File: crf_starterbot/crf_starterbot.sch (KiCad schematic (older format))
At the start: 49 parts, among them J101 Screw_Terminal_01x02, J102 Conn_01x10_Female, J103 Screw_Terminal_01x02, J104 Screw_Terminal_01x02, Q101 Q_NPN_BCE, SW101 SW_SPST, SW102 SW_SPST, SW103 SW_SPST, U101 WeMos_D1_mini, U102 HC-SR04, U103 LM393, U104 E048-03, U106 E048-03, U107 L9110, U108 L9110

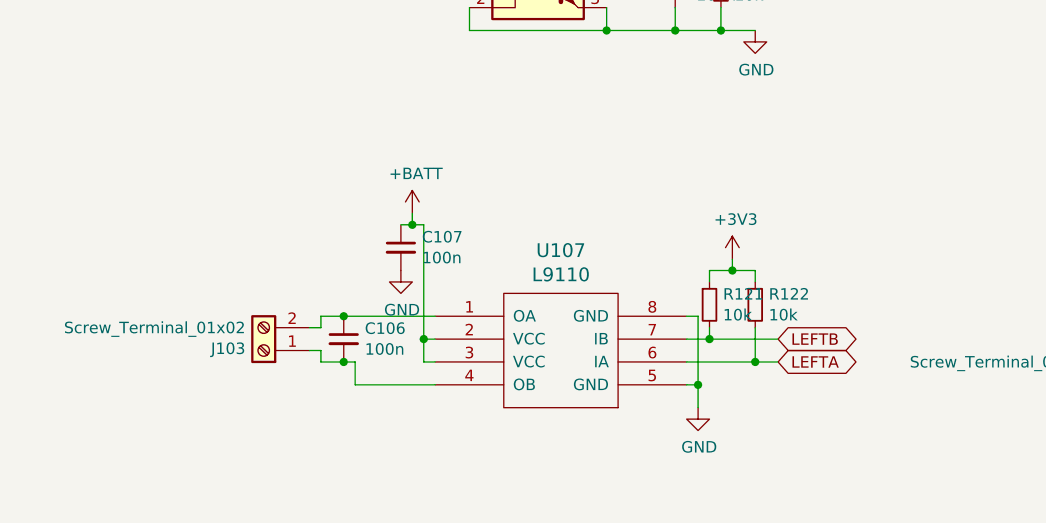
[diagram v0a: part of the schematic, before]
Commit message: Started layout considerations of the pcb
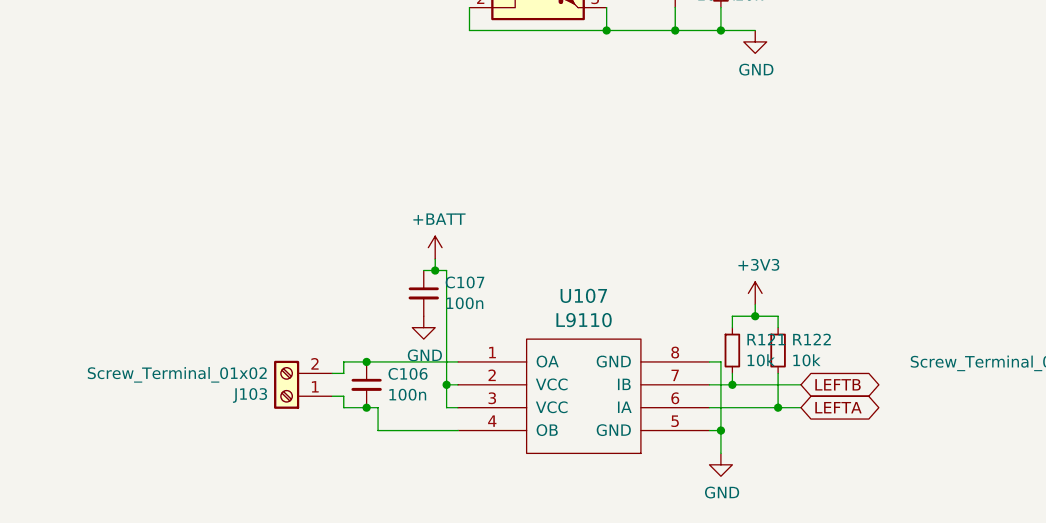
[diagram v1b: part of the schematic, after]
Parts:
- U102: footprint XCVR_HC-SR04 -> Connector_PinHeader_2.54mm:PinHeader_1x04_P2.54mm_Vertical
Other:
- moved on the sheet: C106, C107, J103, R121, R122, U107
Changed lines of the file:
@@
 L Connector:Screw_Terminal_01x02 J103
 U 1 1 5D6CCB3D
-P 800 6750
-F 0 "J103" H 880 6742 50  0000 L CNN
-F 1 "Screw_Terminal_01x02" H 880 6651 50  0000 L CNN
-F 2 "TerminalBlock_Phoenix:TerminalBlock_Phoenix_MKDS-1,5-2_1x02_P5.00mm_Horizontal" H 800 6750 50  0001 C CNN
-F 3 "~" H 800 6750 50  0001 C CNN
-	1    800  6750
+P 900 6950
+F 0 "J103" H 980 6942 50  0000 L CNN
+F 1 "Screw_Terminal_01x02" H 980 6851 50  0000 L CNN
+F 2 "TerminalBlock_Phoenix:TerminalBlock_Phoenix_MKDS-1,5-2_1x02_P5.00mm_Horizontal" H 900 6950 50  0001 C CNN
+F 3 "~" H 900 6950 50  0001 C CNN
+	1    900  6950
 	-1   0    0    1
 $EndComp
@@
 F 0 "U102" H 9980 1696 50  0000 L CNN
 F 1 "HC-SR04" H 9980 1605 50  0000 L CNN
-F 2 "XCVR_HC-SR04" H 9550 1700 50  0001 L BNN
+F 2 "Connector_PinHeader_2.54mm:PinHeader_1x04_P2.54mm_Vertical" H 9550 1700 50  0001 L BNN
 F 3 "Unavailable" H 9550 1700 50  0001 L BNN
 F 4 "HC-SR04 Ultrasonic Sensor For Arduino And Raspberry Pi HC-SR04 Ultrasonic Sensor For Arduino And Raspberry Pi" H 9550 1700 50  0001 L BNN "Field4"
@@
 L crf_starterbot-rescue:L9110-motordriver U107
 U 1 1 5D73C910
-P 2100 6750
-F 0 "U107" H 2100 7187 60  0000 C CNN
-F 1 "L9110" H 2100 7081 60  0000 C CNN
-F 2 "Package_DIP:DIP-8_W7.62mm_Socket" H 2100 6750 60  0001 C CNN
-F 3 "" H 2100 6750 60  0000 C CNN
-	1    2100 6750
+P 2200 6950
+F 0 "U107" H 2200 7387 60  0000 C CNN
+F 1 "L9110" H 2200 7281 60  0000 C CNN
+F 2 "Package_DIP:DIP-8_W7.62mm_Socket" H 2200 6950 60  0001 C CNN
+F 3 "" H 2200 6950 60  0000 C CNN
+	1    2200 6950
 	1    0    0    -1
 $EndComp
@@
 L Device:C_Small C106
 U 1 1 5D6E812A
-P 1150 6700
-F 0 "C106" H 1242 6746 50  0000 L CNN
-F 1 "100n" H 1242 6655 50  0000 L CNN
-F 2 "Capacitor_THT:C_Disc_D5.0mm_W2.5mm_P5.00mm" H 1150 6700 50  0001 C CNN
-F 3 "~" H 1150 6700 50  0001 C CNN
-	1    1150 6700
-	1    0    0    -1
-$EndComp
-Wire Wire Line
-	1550 6800 1500 6800
-Wire Wire Line
-	1500 6800 1500 6700
-Wire Wire Line
-	1500 6700 1550 6700
-Connection ~ 1500 6700
-Wire Wire Line
-	1000 6650 1050 6650
-Wire Wire Line
-	1050 6650 1050 6600
-Wire Wire Line
-	1050 6600 1150 6600
-Wire Wire Line
-	1000 6750 1050 6750
-Wire Wire Line
-	1050 6750 1050 6800
-Wire Wire Line
-	1050 6800 1150 6800
-Wire Wire Line
-	1150 6800 1200 6800
-Wire Wire Line
-	1200 6800 1200 6900
-Wire Wire Line
-	1200 6900 1550 6900
-Connection ~ 1150 6800
-Wire Wire Line
-	1550 6600 1150 6600
-Connection ~ 1150 6600
-Wire Wire Line
-	2650 6600 2700 6600
-Wire Wire Line
-	2700 6600 2700 6900
-Wire Wire Line
-	2700 6900 2650 6900
-Wire Wire Line
-	2700 6900 2700 7000
-Connection ~ 2700 6900
+P 1250 6900
+F 0 "C106" H 1342 6946 50  0000 L CNN
+F 1 "100n" H 1342 6855 50  0000 L CNN
+F 2 "Capacitor_THT:C_Disc_D5.0mm_W2.5mm_P5.00mm" H 1250 6900 50  0001 C CNN
+F 3 "~" H 1250 6900 50  0001 C CNN
+	1    1250 6900
+	1    0    0    -1
+$EndComp
+Wire Wire Line
+	1650 7000 1600 7000
+Wire Wire Line
+	1600 7000 1600 6900
+Wire Wire Line
+	1600 6900 1650 6900
+Connection ~ 1600 6900
+Wire Wire Line
+	1100 6850 1150 6850
+Wire Wire Line
+	1150 6850 1150 6800
+Wire Wire Line
+	1150 6800 1250 6800
+Wire Wire Line
+	1100 6950 1150 6950
+Wire Wire Line
+	1150 6950 1150 7000
+Wire Wire Line
+	1150 7000 1250 7000
+Wire Wire Line
+	1250 7000 1300 7000
+Wire Wire Line
+	1300 7000 1300 7100
+Wire Wire Line
+	1300 7100 1650 7100
+Connection ~ 1250 7000
+Wire Wire Line
+	1650 6800 1250 6800
+Connection ~ 1250 6800
+Wire Wire Line
+	2750 6800 2800 6800
+Wire Wire Line
+	2800 6800 2800 7100
+Wire Wire Line
+	2800 7100 2750 7100
+Wire Wire Line
+	2800 7100 2800 7200
+Connection ~ 2800 7100
 $Comp
 L power:GND #PWR0129
 U 1 1 5D6F59BE
-P 2700 7000
-F 0 "#PWR0129" H 2700 6750 50  0001 C CNN
-F 1 "GND" H 2705 6827 50  0000 C CNN
-F 2 "" H 2700 7000 50  0001 C CNN
-F 3 "" H 2700 7000 50  0001 C CNN
-	1    2700 7000
-	1    0    0    -1
-$EndComp
-Wire Wire Line
-	2650 6700 2750 6700
-Wire Wire Line
-	2650 6800 2950 6800
-Text GLabel 3050 6700 2    50   BiDi ~ 0
+P 2800 7200
+F 0 "#PWR0129" H 2800 6950 50  0001 C CNN
+F 1 "GND" H 2805 7027 50  0000 C CNN
+F 2 "" H 2800 7200 50  0001 C CNN
+F 3 "" H 2800 7200 50  0001 C CNN
+	1    2800 7200
+	1    0    0    -1
+$EndComp
+Wire Wire Line
+	2750 6900 2850 6900
+Wire Wire Line
+	2750 7000 3050 7000
+Text GLabel 3150 6900 2    50   BiDi ~ 0
 LEFTB
-Text GLabel 3050 6800 2    50   BiDi ~ 0
+Text GLabel 3150 7000 2    50   BiDi ~ 0
 LEFTA
 $Comp
 L Device:R_Small R121
 U 1 1 5D6FEF2D
-P 2750 6550
-F 0 "R121" H 2809 6596 50  0000 L CNN
-F 1 "10k" H 2809 6505 50  0000 L CNN
-F 2 "Resistor_THT:R_Axial_DIN0207_L6.3mm_D2.5mm_P7.62mm_Horizontal" H 2750 6550 50  0001 C CNN
-F 3 "~" H 2750 6550 50  0001 C CNN
-	1    2750 6550
+P 2850 6750
+F 0 "R121" H 2909 6796 50  0000 L CNN
+F 1 "10k" H 2909 6705 50  0000 L CNN
+F 2 "Resistor_THT:R_Axial_DIN0207_L6.3mm_D2.5mm_P7.62mm_Horizontal" H 2850 6750 50  0001 C CNN
+F 3 "~" H 2850 6750 50  0001 C CNN
+	1    2850 6750
 	1    0    0    -1
 $EndComp
@@
 L Device:R_Small R122
 U 1 1 5D6FF8E2
-P 2950 6550
-F 0 "R122" H 3009 6596 50  0000 L CNN
-F 1 "10k" H 3009 6505 50  0000 L CNN
-F 2 "Resistor_THT:R_Axial_DIN0207_L6.3mm_D2.5mm_P7.62mm_Horizontal" H 2950 6550 50  0001 C CNN
-F 3 "~" H 2950 6550 50  0001 C CNN
-	1    2950 6550
-	1    0    0    -1
-$EndComp
-Wire Wire Line
-	2750 6650 2750 6700
-Connection ~ 2750 6700
-Wire Wire Line
-	2750 6700 3050 6700
-Wire Wire Line
-	2950 6650 2950 6800
-Connection ~ 2950 6800
-Wire Wire Line
-	2950 6800 3050 6800
-Wire Wire Line
-	2750 6450 2750 6400
-Wire Wire Line
-	2750 6400 2850 6400
-Wire Wire Line
-	2950 6400 2950 6450
-Wire Wire Line
-	2850 6350 2850 6400
-Connection ~ 2850 6400
-Wire Wire Line
-	2850 6400 2950 6400
+P 3050 6750
+F 0 "R122" H 3109 6796 50  0000 L CNN
+F 1 "10k" H 3109 6705 50  0000 L CNN
+F 2 "Resistor_THT:R_Axial_DIN0207_L6.3mm_D2.5mm_P7.62mm_Horizontal" H 3050 6750 50  0001 C CNN
+F 3 "~" H 3050 6750 50  0001 C CNN
+	1    3050 6750
+	1    0    0    -1
+$EndComp
+Wire Wire Line
+	2850 6850 2850 6900
+Connection ~ 2850 6900
+Wire Wire Line
+	2850 6900 3150 6900
+Wire Wire Line
+	3050 6850 3050 7000
+Connection ~ 3050 7000
+Wire Wire Line
+	3050 7000 3150 7000
+Wire Wire Line
+	2850 6650 2850 6600
+Wire Wire Line
+	2850 6600 2950 6600
+Wire Wire Line
+	3050 6600 3050 6650
+Wire Wire Line
+	2950 6550 2950 6600
+Connection ~ 2950 6600
+Wire Wire Line
+	2950 6600 3050 6600
 $Comp
 L power:+3V3 #PWR0130
 U 1 1 5D70A877
-P 2850 6350
-F 0 "#PWR0130" H 2850 6200 50  0001 C CNN
-F 1 "+3V3" H 2865 6523 50  0000 C CNN
-F 2 "" H 2850 6350 50  0001 C CNN
-F 3 "" H 2850 6350 50  0001 C CNN
-	1    2850 6350
+P 2950 6550
+F 0 "#PWR0130" H 2950 6400 50  0001 C CNN
+F 1 "+3V3" H 2965 6723 50  0000 C CNN
+F 2 "" H 2950 6550 50  0001 C CNN
+F 3 "" H 2950 6550 50  0001 C CNN
+	1    2950 6550
 	1    0    0    -1
 $EndComp
@@
 L Device:C_Small C107
 U 1 1 5D70B833
-P 1400 6300
-F 0 "C107" H 1492 6346 50  0000 L CNN
-F 1 "100n" H 1492 6255 50  0000 L CNN
-F 2 "Capacitor_THT:C_Disc_D5.0mm_W2.5mm_P5.00mm" H 1400 6300 50  0001 C CNN
-F 3 "~" H 1400 6300 50  0001 C CNN
-	1    1400 6300
+P 1500 6500
+F 0 "C107" H 1592 6546 50  0000 L CNN
+F 1 "100n" H 1592 6455 50  0000 L CNN
+F 2 "Capacitor_THT:C_Disc_D5.0mm_W2.5mm_P5.00mm" H 1500 6500 50  0001 C CNN
+F 3 "~" H 1500 6500 50  0001 C CNN
+	1    1500 6500
 	1    0    0    -1
 $EndComp
@@
 L power:GND #PWR0127
 U 1 1 5D70DE8A
-P 1400 6400
-F 0 "#PWR0127" H 1400 6150 50  0001 C CNN
-F 1 "GND" H 1405 6227 50  0000 C CNN
-F 2 "" H 1400 6400 50  0001 C CNN
-F 3 "" H 1400 6400 50  0001 C CNN
-	1    1400 6400
+P 1500 6600
+F 0 "#PWR0127" H 1500 6350 50  0001 C CNN
+F 1 "GND" H 1505 6427 50  0000 C CNN
+F 2 "" H 1500 6600 50  0001 C CNN
+F 3 "" H 1500 6600 50  0001 C CNN
+	1    1500 6600
 	1    0    0    -1
 $EndComp
@@
 L power:+BATT #PWR0128
 U 1 1 5D70E7D9
-P 1450 6150
-F 0 "#PWR0128" H 1450 6000 50  0001 C CNN
-F 1 "+BATT" H 1465 6323 50  0000 C CNN
-F 2 "" H 1450 6150 50  0001 C CNN
-F 3 "" H 1450 6150 50  0001 C CNN
-	1    1450 6150
-	1    0    0    -1
-$EndComp
-Wire Wire Line
-	1400 6200 1450 6200
-Wire Wire Line
-	1450 6200 1450 6150
-Wire Wire Line
-	1450 6200 1500 6200
-Wire Wire Line
-	1500 6200 1500 6700
-Connection ~ 1450 6200
+P 1550 6350
+F 0 "#PWR0128" H 1550 6200 50  0001 C CNN
+F 1 "+BATT" H 1565 6523 50  0000 C CNN
+F 2 "" H 1550 6350 50  0001 C CNN
+F 3 "" H 1550 6350 50  0001 C CNN
+	1    1550 6350
+	1    0    0    -1
+$EndComp
+Wire Wire Line
+	1500 6400 1550 6400
+Wire Wire Line
+	1550 6400 1550 6350
+Wire Wire Line
+	1550 6400 1600 6400
+Wire Wire Line
+	1600 6400 1600 6900
+Connection ~ 1550 6400
 $Comp
 L Connector:Screw_Terminal_01x02 J104
